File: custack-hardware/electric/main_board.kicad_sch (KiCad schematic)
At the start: 33 parts, among them J2 Conn_01x02, J3 Conn_02x15_Odd_Even, J4 Conn_01x04, J5 Conn_01x04, J6 Conn_01x04, Q2 Q_NMOS, U1 TPS562200DDCR

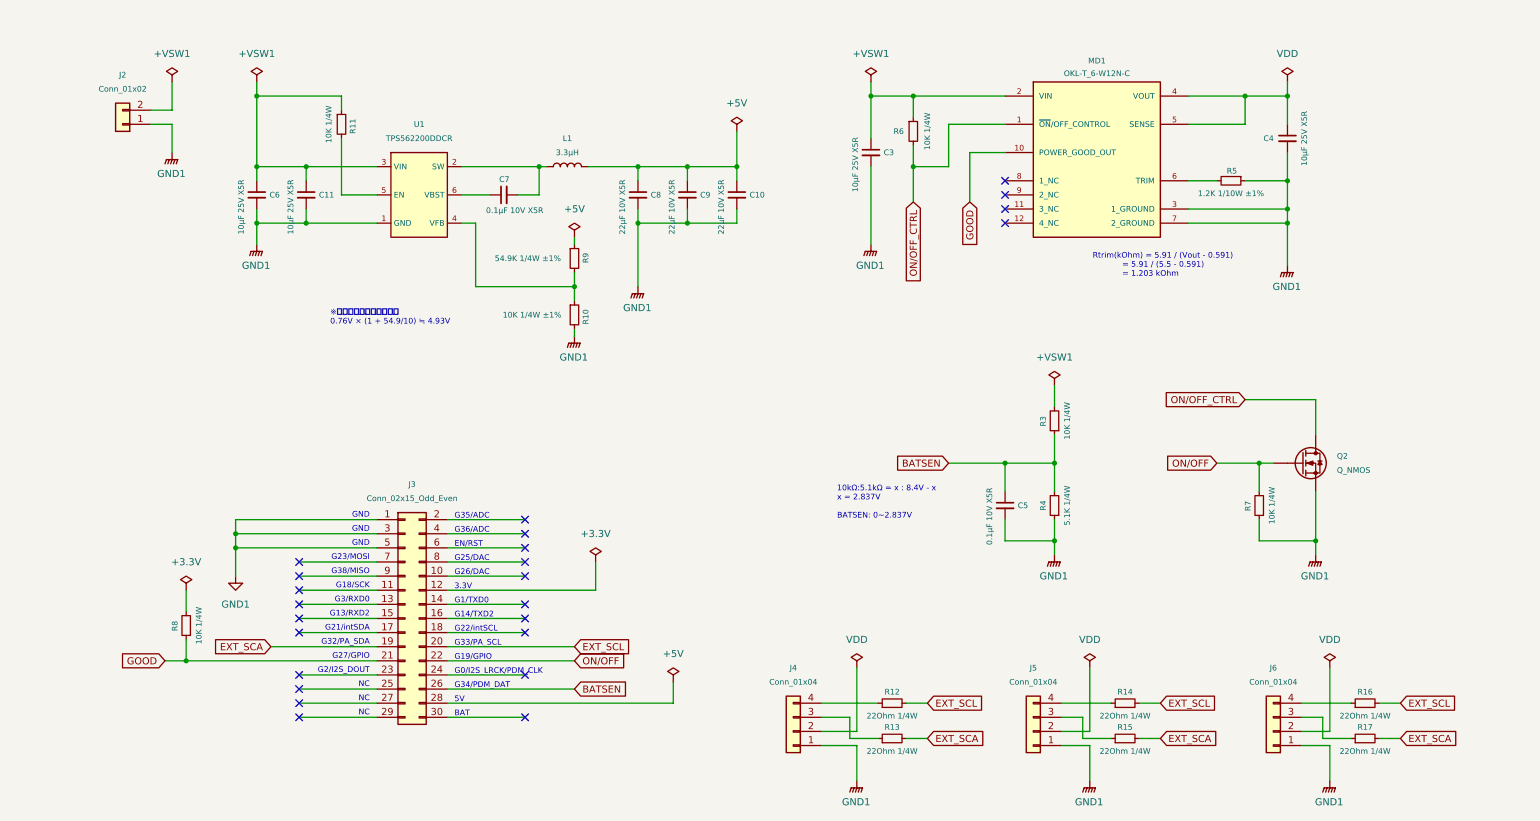
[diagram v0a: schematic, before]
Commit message: 型番確定作業途中
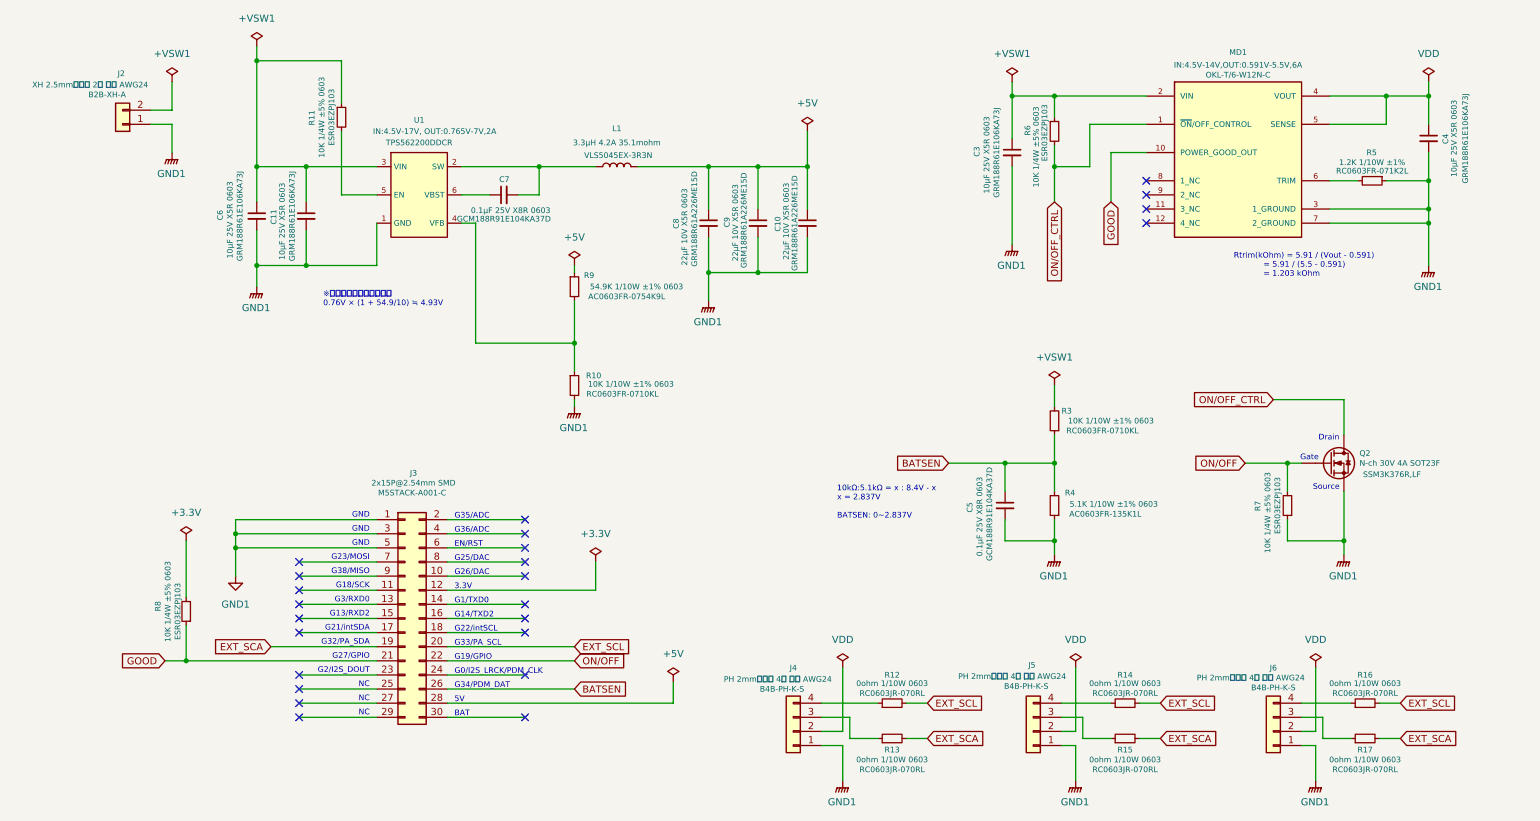
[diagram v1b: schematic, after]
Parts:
- C10, C8, C9: value 22µF 10V X5R -> 22µF 10V X5R 0603; footprint (none) -> Capacitor_SMD:C_0603_1608Metric; 型式 (none) -> GRM188R61A226ME15D
- C11, C3, C4, C6: value 10µF 25V X5R -> 10µF 25V X5R 0603; footprint (none) -> Capacitor_SMD:C_0603_1608Metric; 型式 (none) -> GRM188R61E106KA73J
- C5, C7: value 0.1µF 10V X5R -> 0.1µF 25V X8R 0603; footprint (none) -> Capacitor_SMD:C_0603_1608Metric; 型式 (none) -> GCM188R91E104KA37D
- J2: value Conn_01x02 -> XH 2.5mmピッチ 2極 オス AWG24; footprint (none) -> Connector_JST:JST_XH_B2B-XH-A_1x02_P2.50mm_Vertical; 型式 (none) -> B2B-XH-A
- J3: value Conn_02x15_Odd_Even -> 2x15P@2.54mm SMD; footprint (none) -> My_Custom:M5Stack_Bus_Socket; 型式 (none) -> M5STACK-A001-C
- J4, J5, J6: value Conn_01x04 -> PH 2mmピッチ 4極 オス AWG24; footprint (none) -> Connector_JST:JST_PH_B4B-PH-K_1x04_P2.00mm_Vertical; 型式 (none) -> B4B-PH-K-S
- L1: value 3.3µH -> 3.3µH 4.2A 35.1mohm; footprint (none) -> My_Custom:IND_VLS5045EX-3R3N; 型式 (none) -> VLS5045EX-3R3N
- MD1: value OKL-T_6-W12N-C -> IN:4.5V-14V,OUT:0.591V-5.5V,6A; footprint OKL-T_6-W12N-C:MURATA_OKL-T-6-W12N-C_0 -> My_Custom:MURATA_OKL-T-6-W12N-C_0; 型式 (none) -> OKL-T/6-W12N-C
- Q2: value Q_NMOS -> N-ch 30V 4A SOT23F; footprint (none) -> Package_TO_SOT_SMD:SOT-23; 型式 (none) -> SSM3K376R,LF
- R10: value 10K 1/4W ±1% -> 10K 1/10W ±1% 0603; footprint (none) -> Resistor_SMD:R_0603_1608Metric; 型式 (none) -> RC0603FR-0710KL
- R11, R6, R7, R8: value 10K 1/4W -> 10K 1/4W ±5% 0603; footprint (none) -> Resistor_SMD:R_0603_1608Metric; 型式 (none) -> ESR03EZPJ103
- R12, R13, R14, R15, R16, R17: value 22Ohm 1/4W -> 0ohm 1/10W 0603; footprint (none) -> Resistor_SMD:R_0603_1608Metric; 型式 (none) -> RC0603JR-070RL
- R3: value 10K 1/4W -> 10K 1/10W ±1% 0603; footprint (none) -> Resistor_SMD:R_0603_1608Metric; 型式 (none) -> RC0603FR-0710KL
- R4: value 5.1K 1/4W -> 5.1K 1/10W ±1% 0603; footprint (none) -> Resistor_SMD:R_0603_1608Metric; 型式 (none) -> AC0603FR-135K1L
- R5: footprint (none) -> Resistor_SMD:R_0603_1608Metric; 型式 (none) -> RC0603FR-071K2L
- R9: value 54.9K 1/4W ±1% -> 54.9K 1/10W ±1% 0603; footprint (none) -> Resistor_SMD:R_0603_1608Metric; 型式 (none) -> AC0603FR-0754K9L
- U1: value TPS562200DDCR -> IN:4.5V-17V, OUT:0.765V-7V,2A
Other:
- note added: "Drain"
- note added: "Gate"
- note added: "Source"
- moved on the sheet: C10, C11, C3, C4, C6, C8, C9, L1, MD1, Q2, R10, R11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

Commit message: electric circut complete
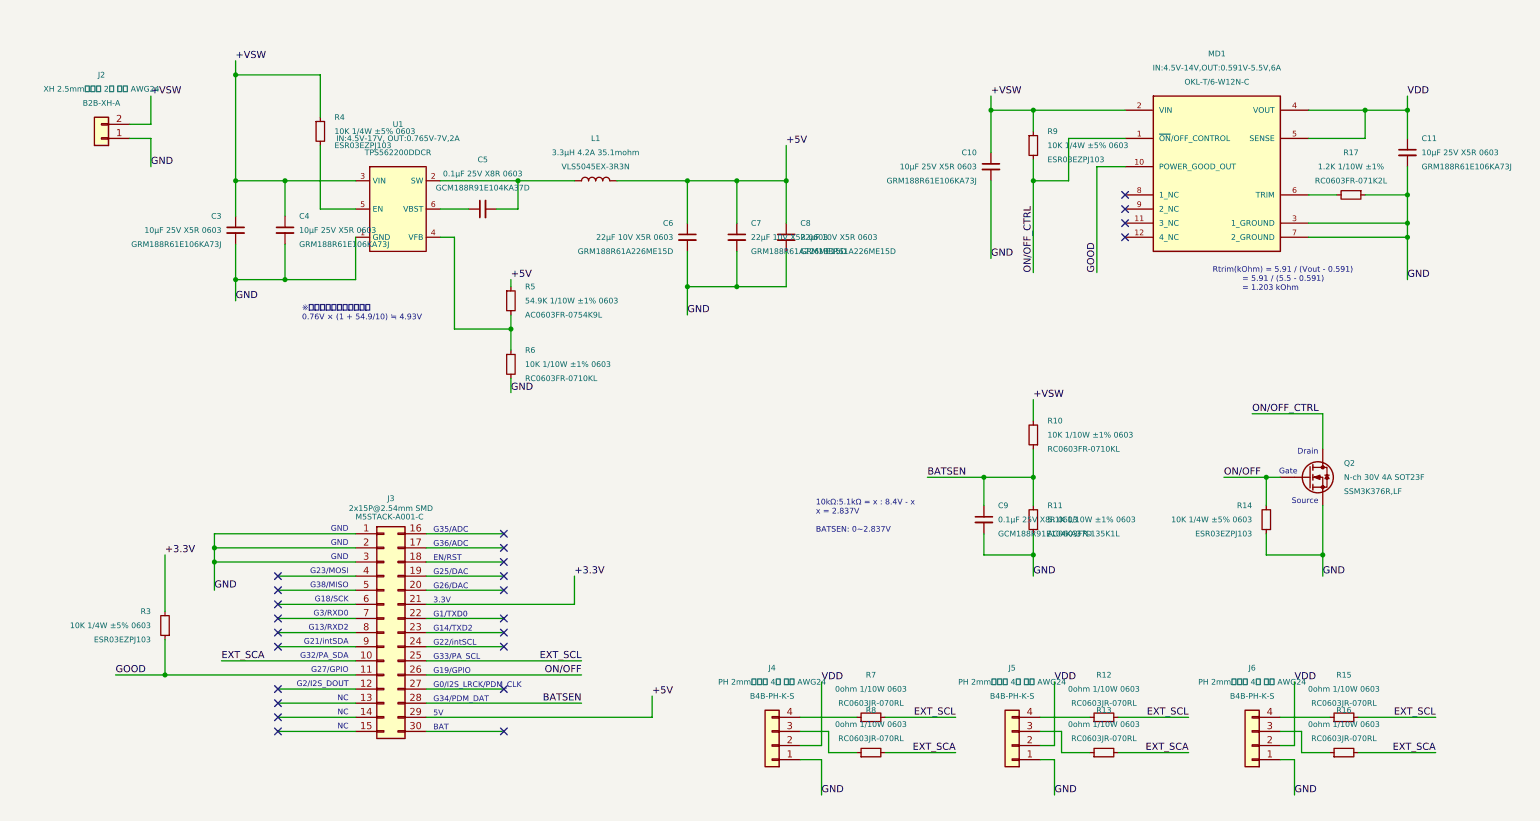
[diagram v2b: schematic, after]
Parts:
- removed J3: 2x15P@2.54mm SMD, My_Custom:M5Stack_Bus_Socket, symbol My_Connector_Generic:Conn_02x15_Odd_Even
- added J3: 2x15P@2.54mm SMD, My_Custom:M5Stack_Bus_Socket, symbol My_Connector_Generic:Conn_02x15_Top_Bottom
- C10: value 22µF 10V X5R 0603 -> 10µF 25V X5R 0603; 型式 GRM188R61A226ME15D -> GRM188R61E106KA73J
- C6: value 10µF 25V X5R 0603 -> 22µF 10V X5R 0603; 型式 GRM188R61E106KA73J -> GRM188R61A226ME15D
- C7: value 0.1µF 25V X8R 0603 -> 22µF 10V X5R 0603; 型式 GCM188R91E104KA37D -> GRM188R61A226ME15D
- C9: value 22µF 10V X5R 0603 -> 0.1µF 25V X8R 0603; 型式 GRM188R61A226ME15D -> GCM188R91E104KA37D
- R11: value 10K 1/4W ±5% 0603 -> 5.1K 1/10W ±1% 0603; 型式 ESR03EZPJ103 -> AC0603FR-135K1L
- R14: value 0ohm 1/10W 0603 -> 10K 1/4W ±5% 0603; 型式 RC0603JR-070RL -> ESR03EZPJ103
- R17: value 0ohm 1/10W 0603 -> 1.2K 1/10W ±1%; 型式 RC0603JR-070RL -> RC0603FR-071K2L
- R3: value 10K 1/10W ±1% 0603 -> 10K 1/4W ±5% 0603; 型式 RC0603FR-0710KL -> ESR03EZPJ103
- R4: value 5.1K 1/10W ±1% 0603 -> 10K 1/4W ±5% 0603; 型式 AC0603FR-135K1L -> ESR03EZPJ103
- R5: value 1.2K 1/10W ±1% -> 54.9K 1/10W ±1% 0603; 型式 RC0603FR-071K2L -> AC0603FR-0754K9L
- R6: value 10K 1/4W ±5% 0603 -> 10K 1/10W ±1% 0603; 型式 ESR03EZPJ103 -> RC0603FR-0710KL
- R7, R8: value 10K 1/4W ±5% 0603 -> 0ohm 1/10W 0603; 型式 ESR03EZPJ103 -> RC0603JR-070RL
- R9: value 54.9K 1/10W ±1% 0603 -> 10K 1/4W ±5% 0603; 型式 AC0603FR-0754K9L -> ESR03EZPJ103
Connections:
- net BATSEN: now also C9.1, R10.1, R11.2, J3.28 (Pin_28); no longer C5.1, R3.1, R4.2
- net EXT_SCA: now also R16.2, R8.2, J3.10 (Pin_10); no longer R15.2, R17.2
- net EXT_SCL: now also R15.2, R7.2, J3.25 (Pin_25); no longer R14.2, R16.2
- net GOOD: now also R3.1, J3.11 (Pin_11); no longer R8.1
- net ON/OFF: now also Q2.1 (G), R14.2, J3.26 (Pin_26); no longer Q2.G, R7.2
- net ON/OFF_CTRL: now also Q2.3 (D), R9.2; no longer Q2.D, R6.2
- net VDD: now reaches MD1.4 (VOUT), MD1.5 (SENSE)
- net VDD: now also C11.1, J4.2 (Pin_2), J5.2 (Pin_2), J6.2 (Pin_2); no longer C4.1
- net at J5.3 (Pin_3): now also R13.1; no longer R15.1
- net at R12.1: now also J5.4 (Pin_4); no longer J4.4 (Pin_4)
- net at J6.3 (Pin_3): now also R16.1; no longer R17.1
- net at J6.4 (Pin_4): now also R15.1; no longer R16.1
- net at U1.5 (EN): now also R4.2; no longer R11.2
- net GND: now reaches R14.1
- net GND: now also C10.2, C11.2, C3.2, C4.2, C6.2, C7.2, C8.2, C9.2, J2.1 (Pin_1), J4.1 (Pin_1), J5.1 (Pin_1), J6.1 (Pin_1), MD1.3 (1_GROUND), MD1.7 (2_GROUND), Q2.2 (S), R11.1, R17.1, R6.2, U1.1 (GND), J3.1 (Pin_1), J3.2 (Pin_2), J3.3 (Pin_3); no longer J5.4 (Pin_4)
- net at L1.1, U1.2 (SW): now also C5.2; no longer C7.2
- net at U1.6 (VBST): now also C5.1; no longer C7.1
- net +VSW: now reaches C3.1, MD1.2 (VIN)
- net +VSW: now also C10.1, C4.1, J2.2 (Pin_2), R10.2, R4.1, R9.1, U1.3 (VIN); no longer R6.1
- net +5V: now reaches C8.1, L1.2
- net +5V: now also C6.1, C7.1, R5.1, J3.29 (Pin_29); no longer C10.1, C9.1
- net at J4.3 (Pin_3): now also R8.1; no longer R13.1
- net +3.3V: now reaches R3.2
- net +3.3V: now also J3.21 (Pin_21)
- net at R5.2: now also R6.1, U1.4 (VFB); no longer MD1.6 (TRIM)
- removed net GND1: C10.2, C11.2, C3.2, C4.2, C5.2, C6.2, C8.2, C9.2, J2.1 (Pin_1), J4.1 (Pin_1), J5.1 (Pin_1), J6.1 (Pin_1), MD1.3 (1_GROUND), MD1.7 (2_GROUND), Q2.S, R10.2, R4.1, R5.1, R7.1, U1.1 (GND)
- new net: MD1.6 (TRIM), R17.2
- new net: J4.4 (Pin_4), R7.1
